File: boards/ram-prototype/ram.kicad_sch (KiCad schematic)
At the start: 29 parts, among them J1 SRAM_Bus

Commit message: Add initial changes to make logic close to final
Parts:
- removed J1: SRAM_Bus, symbol Connector_Generic:Conn_01x16
- added D15, D16, D17, D18, D19, D20, D21, D22: Red, symbol Device:LED_Small
- added J1: SRAM_Bus, symbol Connector_Generic:Conn_01x24
- added J2: Probe, symbol Connector_Generic:Conn_01x12
- added J3: Unused_COL_SEL, symbol Connector_Generic:Conn_01x14
- added R15, R16, R17, R18, R19, R20, R21, R22: 680R, symbol Device:R_Small
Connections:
- net Column Select/A2 is gone; now on net D3: D14.2 (A)
- net Address Decoder/A0: now also D10.2 (A), J1.14 (Pin_14); no longer D5.2 (A)
- net Address Decoder/A1: now also D9.2 (A), J1.15 (Pin_15); no longer D4.2 (A)
- net Control Logic/nCE: now also J1.21 (Pin_21)
- net Control Logic/nOE: now also J1.23 (Pin_23)
- net Control Logic/nWE: now also J1.22 (Pin_22)
- net D0: now also D11.2 (A), J1.13 (Pin_13); no longer D6.2 (A)
- net D1: now also D12.2 (A), J1.12 (Pin_12); no longer D7.2 (A)
- net D2: now also D13.2 (A), J1.11 (Pin_11); no longer D8.2 (A)
- net D3: now also J1.10 (Pin_10); no longer D9.2 (A)
- net D4: now also D15.2 (A), J1.9 (Pin_9); no longer D10.2 (A)
- net D5: now also D16.2 (A), J1.8 (Pin_8); no longer D11.2 (A)
- net D6: now also D17.2 (A), J1.7 (Pin_7); no longer D12.2 (A)
- net D7: now also D18.2 (A), J1.6 (Pin_6); no longer D13.2 (A)
- net GND: now also J1.1 (Pin_1), R15.2, R16.2, R17.2, R18.2, R19.2, R20.2, R21.2, R22.2
- net VCC: now also J1.24 (Pin_24)
- new net: D19.1 (K), R19.1
- new net: D17.1 (K), R17.1
- new net: D22.1 (K), R22.1
- new net: D18.1 (K), R18.1
- new net: D21.1 (K), R21.1
- new net: D15.1 (K), R15.1
- new net: D16.1 (K), R16.1
- new net: D20.1 (K), R20.1
- new net Address Decoder/A2: D8.2 (A), J1.16 (Pin_16)
- new net Address Decoder/A3: D7.2 (A), J1.17 (Pin_17)
- new net Address Decoder/A4: D6.2 (A), J1.18 (Pin_18)
- new net Address Decoder/A5: D5.2 (A), J1.19 (Pin_19)
- new net Address Decoder/A6: D4.2 (A), J1.20 (Pin_20)
- new net COL_SEL_10: J3.9 (Pin_9)
- new net COL_SEL_11: J3.10 (Pin_10)
- new net COL_SEL_12: J3.11 (Pin_11)
- new net COL_SEL_13: J3.12 (Pin_12)
- new net COL_SEL_14: J3.13 (Pin_13)
- new net COL_SEL_15: J3.14 (Pin_14)
- new net COL_SEL_2: J3.1 (Pin_1)
- new net COL_SEL_3: J3.2 (Pin_2)
- new net COL_SEL_4: J3.3 (Pin_3)
- new net COL_SEL_5: J3.4 (Pin_4)
- new net COL_SEL_6: J3.5 (Pin_5)
- new net COL_SEL_7: J3.6 (Pin_6)
- new net COL_SEL_8: J3.7 (Pin_7)
- new net COL_SEL_9: J3.8 (Pin_8)
- new net Column Select/A10: D19.2 (A), J1.5 (Pin_5)
- new net Column Select/A7: D22.2 (A), J1.2 (Pin_2)
- new net Column Select/A8: D21.2 (A), J1.3 (Pin_3)
- new net Column Select/A9: D20.2 (A), J1.4 (Pin_4)
- new net GA0: J2.5 (Pin_5)
- new net GA1: J2.6 (Pin_6)
- new net GA2: J2.7 (Pin_7)
- new net GA3: J2.8 (Pin_8)
- new net GB0: J2.9 (Pin_9)
- new net GB1: J2.10 (Pin_10)
- new net GB2: J2.11 (Pin_11)
- new net GB3: J2.12 (Pin_12)
- new net RS1: J2.1 (Pin_1)
- new net RS2: J2.2 (Pin_2)
- new net RS3: J2.3 (Pin_3)
- new net RS4: J2.4 (Pin_4)
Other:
- sheet Address Decoder ports: added A2, A3, A4, A5, A6, RS1, RS2, RS3, RS4; removed none
- sheet Column Select ports: added A10, A7, A8, A9, COL_SEL_10, COL_SEL_11, COL_SEL_12, COL_SEL_13, COL_SEL_14, COL_SEL_15, COL_SEL_2, COL_SEL_3, COL_SEL_4, COL_SEL_5, COL_SEL_6, COL_SEL_7, COL_SEL_8, COL_SEL_9, GA0, GA1, GA2, GA3, GB0, GB1, GB2, GB3; removed A2

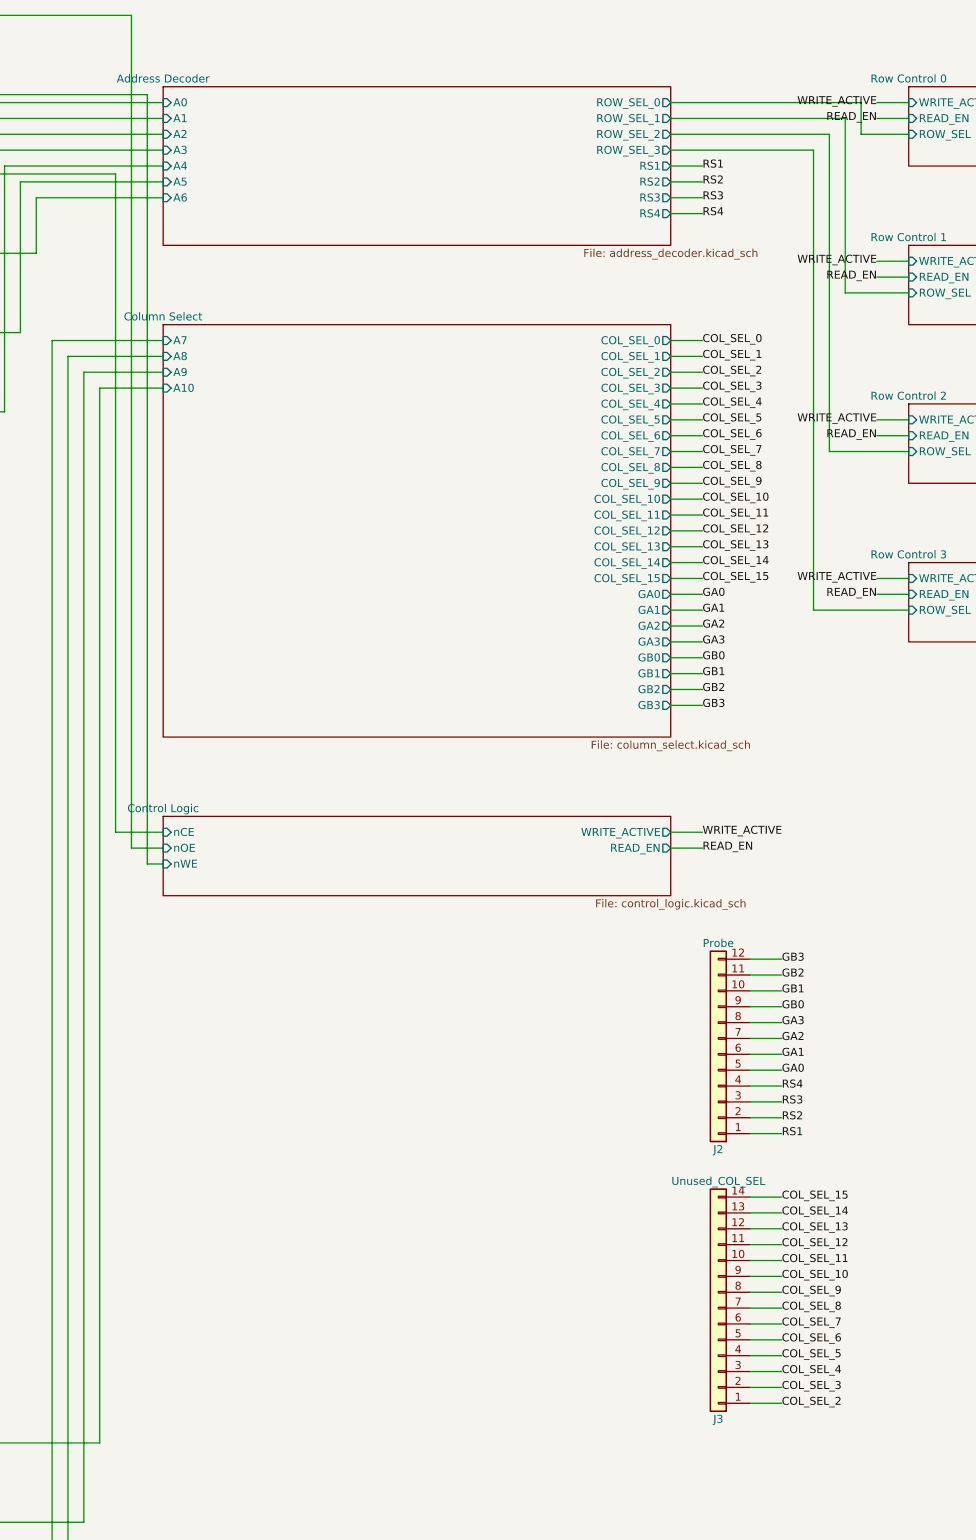
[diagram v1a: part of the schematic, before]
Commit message: clean up
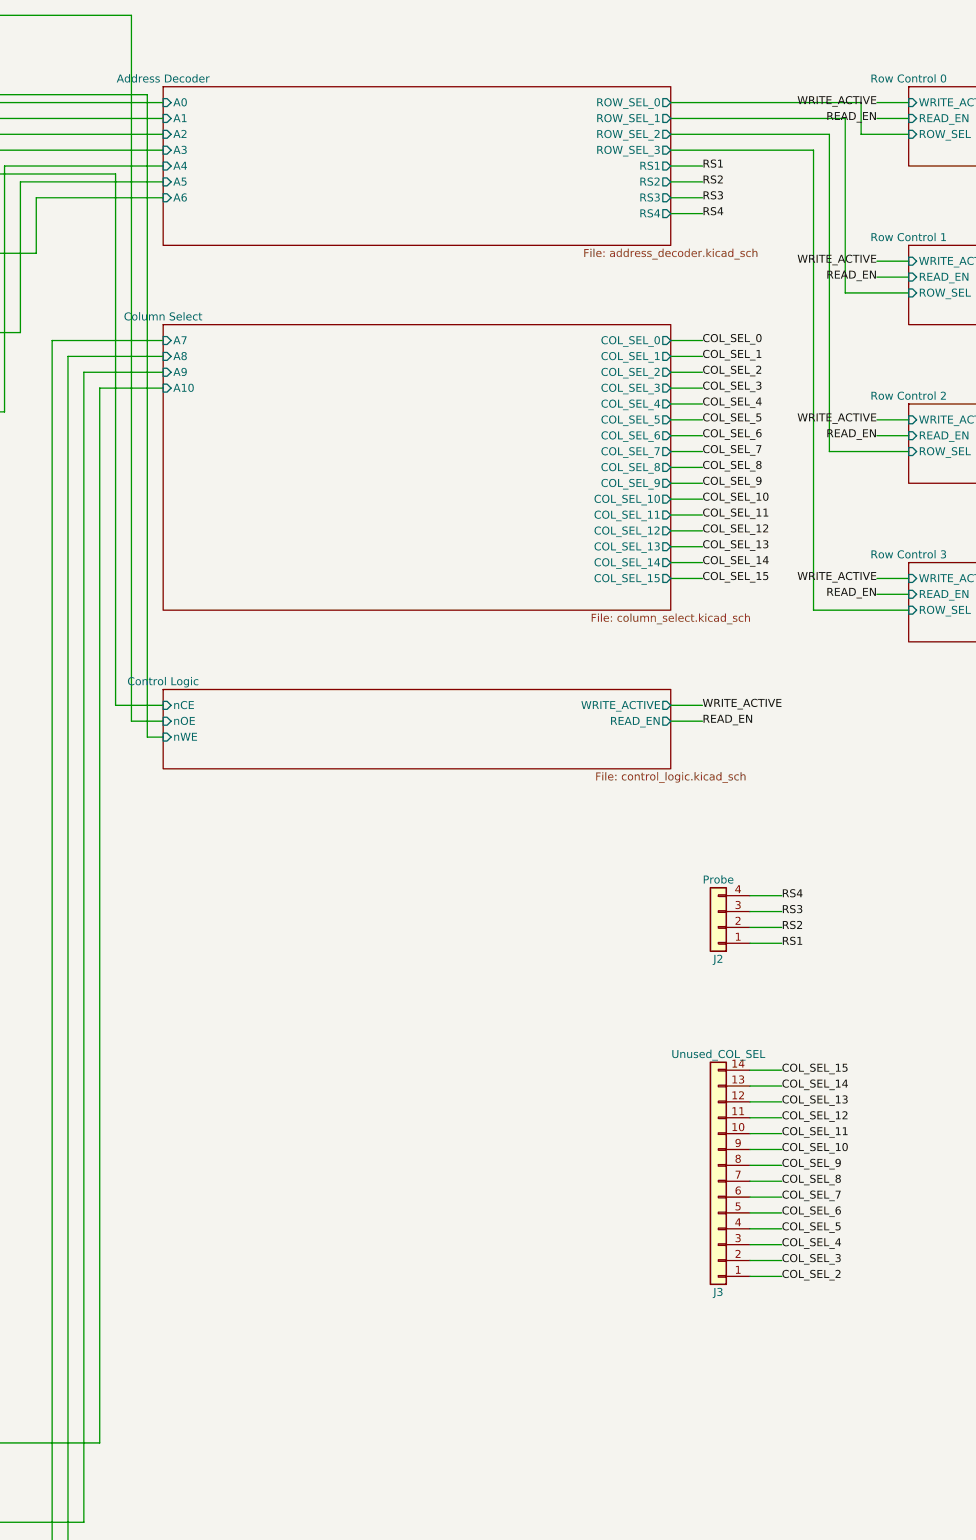
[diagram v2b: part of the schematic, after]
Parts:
- removed J2: Probe, symbol Connector_Generic:Conn_01x12
- added J2: Probe, symbol Connector_Generic:Conn_01x04
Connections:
- net RS1: now also J2.1 (Pin_1)
- net RS2: now also J2.2 (Pin_2)
- net RS3: now also J2.3 (Pin_3)
- net RS4: now also J2.4 (Pin_4)
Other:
- sheet Column Select ports: added none; removed GA0, GA1, GA2, GA3, GB0, GB1, GB2, GB3
